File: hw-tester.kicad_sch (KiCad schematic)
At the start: 51 parts, among them J1 AVR-ISP-6, J10 Conn_01x08, J11 Conn_01x08, J12 Conn_01x08, J13 Conn_01x08, J14 BarrelJack, J15 Conn_01x08, J16 Conn_01x08, J17 Conn_01x08, J18 Conn_01x08, J19 USB_B_Mini, J2 Conn_01x08, J3 Conn_01x08, J4 Conn_01x08, J5 Conn_01x08, J6 Conn_01x08, J7 Conn_01x08, J8 Conn_01x08, J9 Conn_01x08, U15 ATmega324PB-M, U28 FT230XQ, U30 ADuM1201AR, X1 IQXO-70

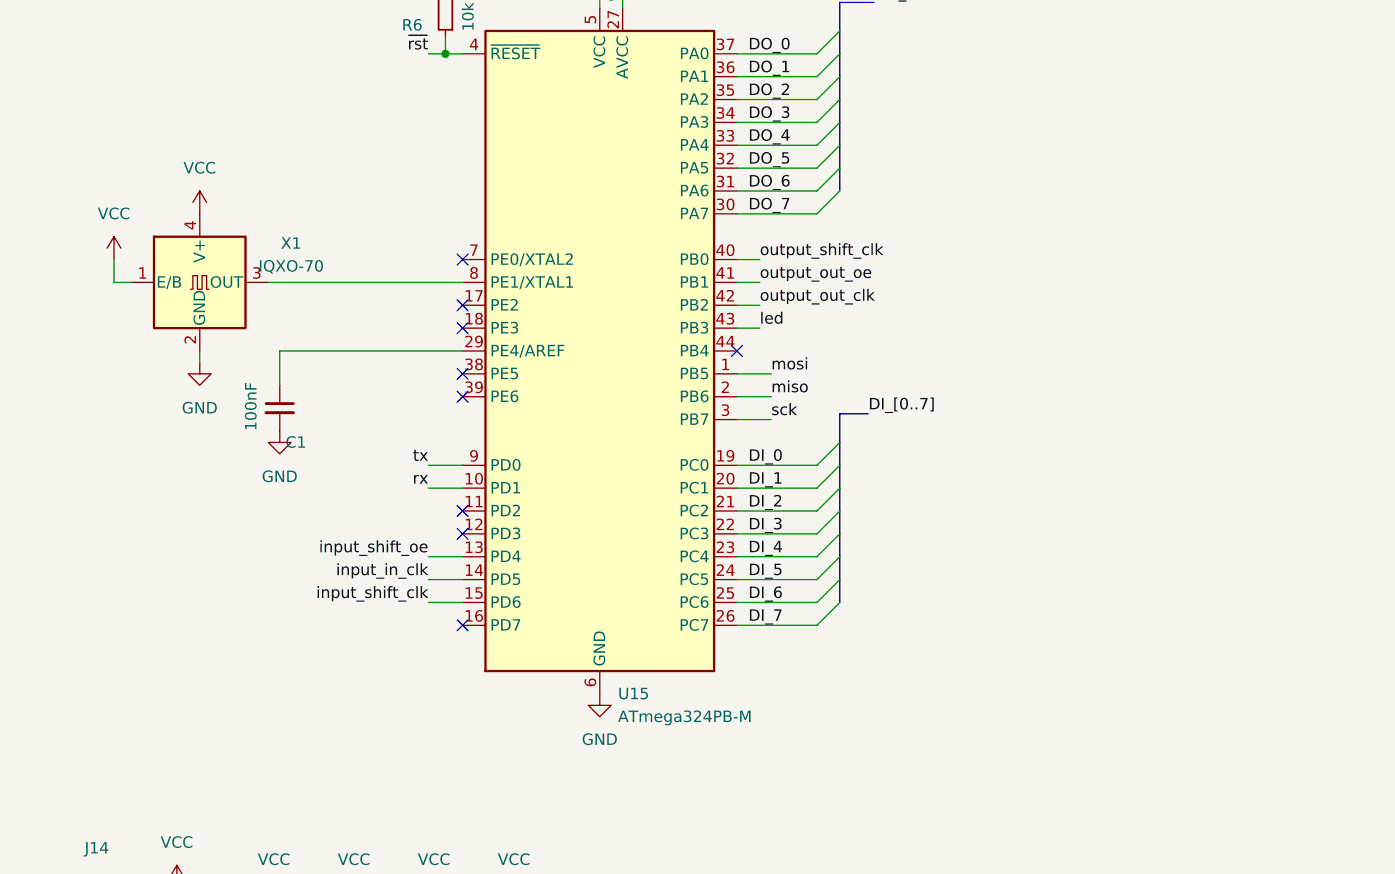
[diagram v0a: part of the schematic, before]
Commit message: firmware
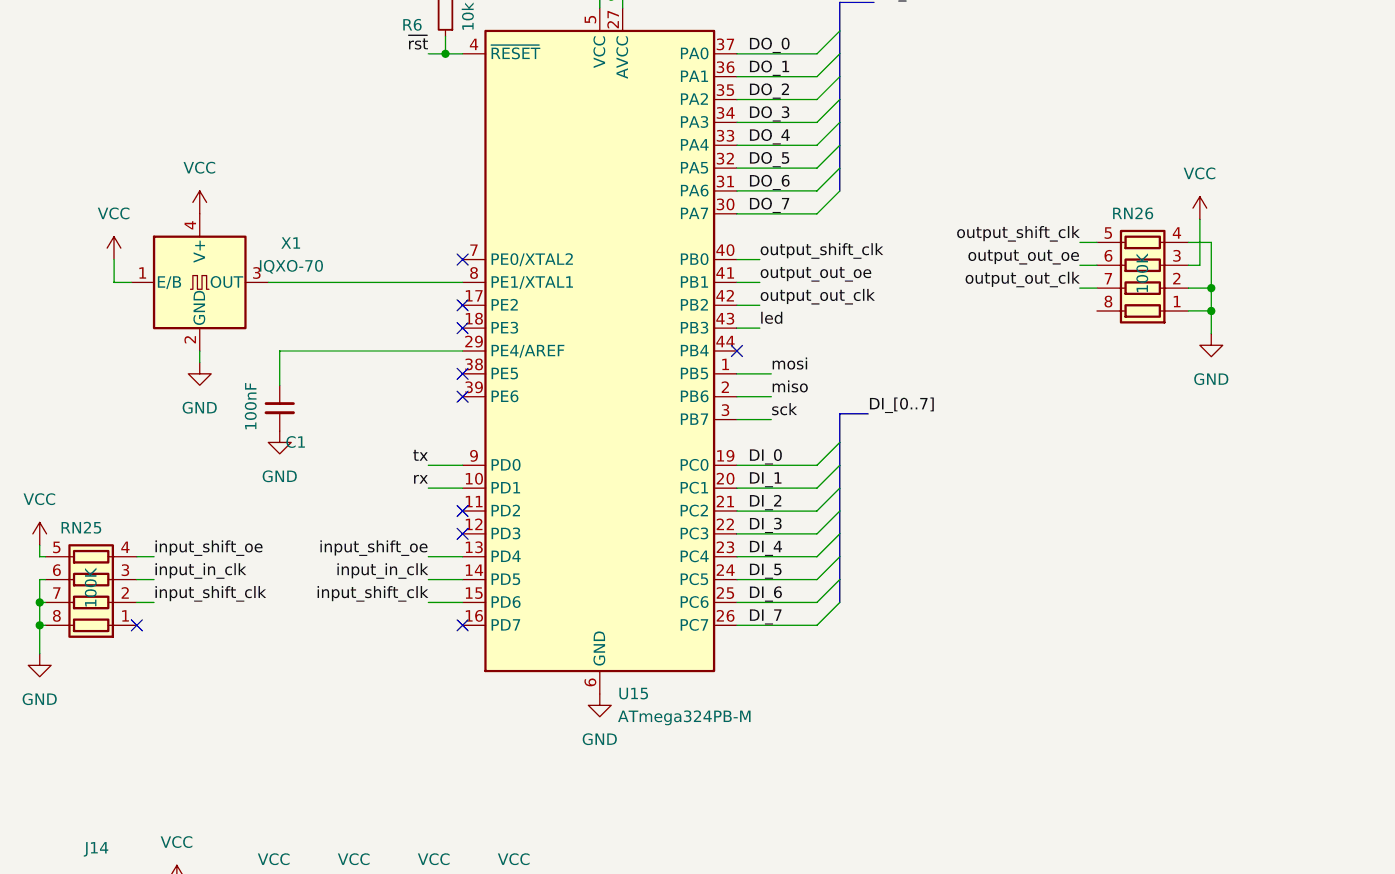
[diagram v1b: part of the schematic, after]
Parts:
- added RN25, RN26: 100K, Resistor_SMD:R_Array_Convex_4x0603, symbol Device:R_Pack04
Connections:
- net GND: now also RN25.6 (R3.2), RN25.7 (R2.2), RN25.8 (R1.2), RN26.1 (R1.1), RN26.2 (R2.1), RN26.4 (R4.1)
- net VCC: now also RN25.5 (R4.2), RN26.3 (R3.1)
- net input_in_clk: now also RN25.3 (R3.1)
- net input_shift_clk: now also RN25.2 (R2.1)
- net input_shift_oe: now also RN25.4 (R4.1)
- net output_out_clk: now also RN26.7 (R2.2)
- net output_out_oe: now also RN26.6 (R3.2)
- net output_shift_clk: now also RN26.5 (R4.2)
- no-connect marks 15 -> 16
